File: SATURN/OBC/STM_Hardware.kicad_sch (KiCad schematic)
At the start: 6 parts, among them J1 SWD Pins, P1 USB_C_Plug, U1 STM32H735AGIx

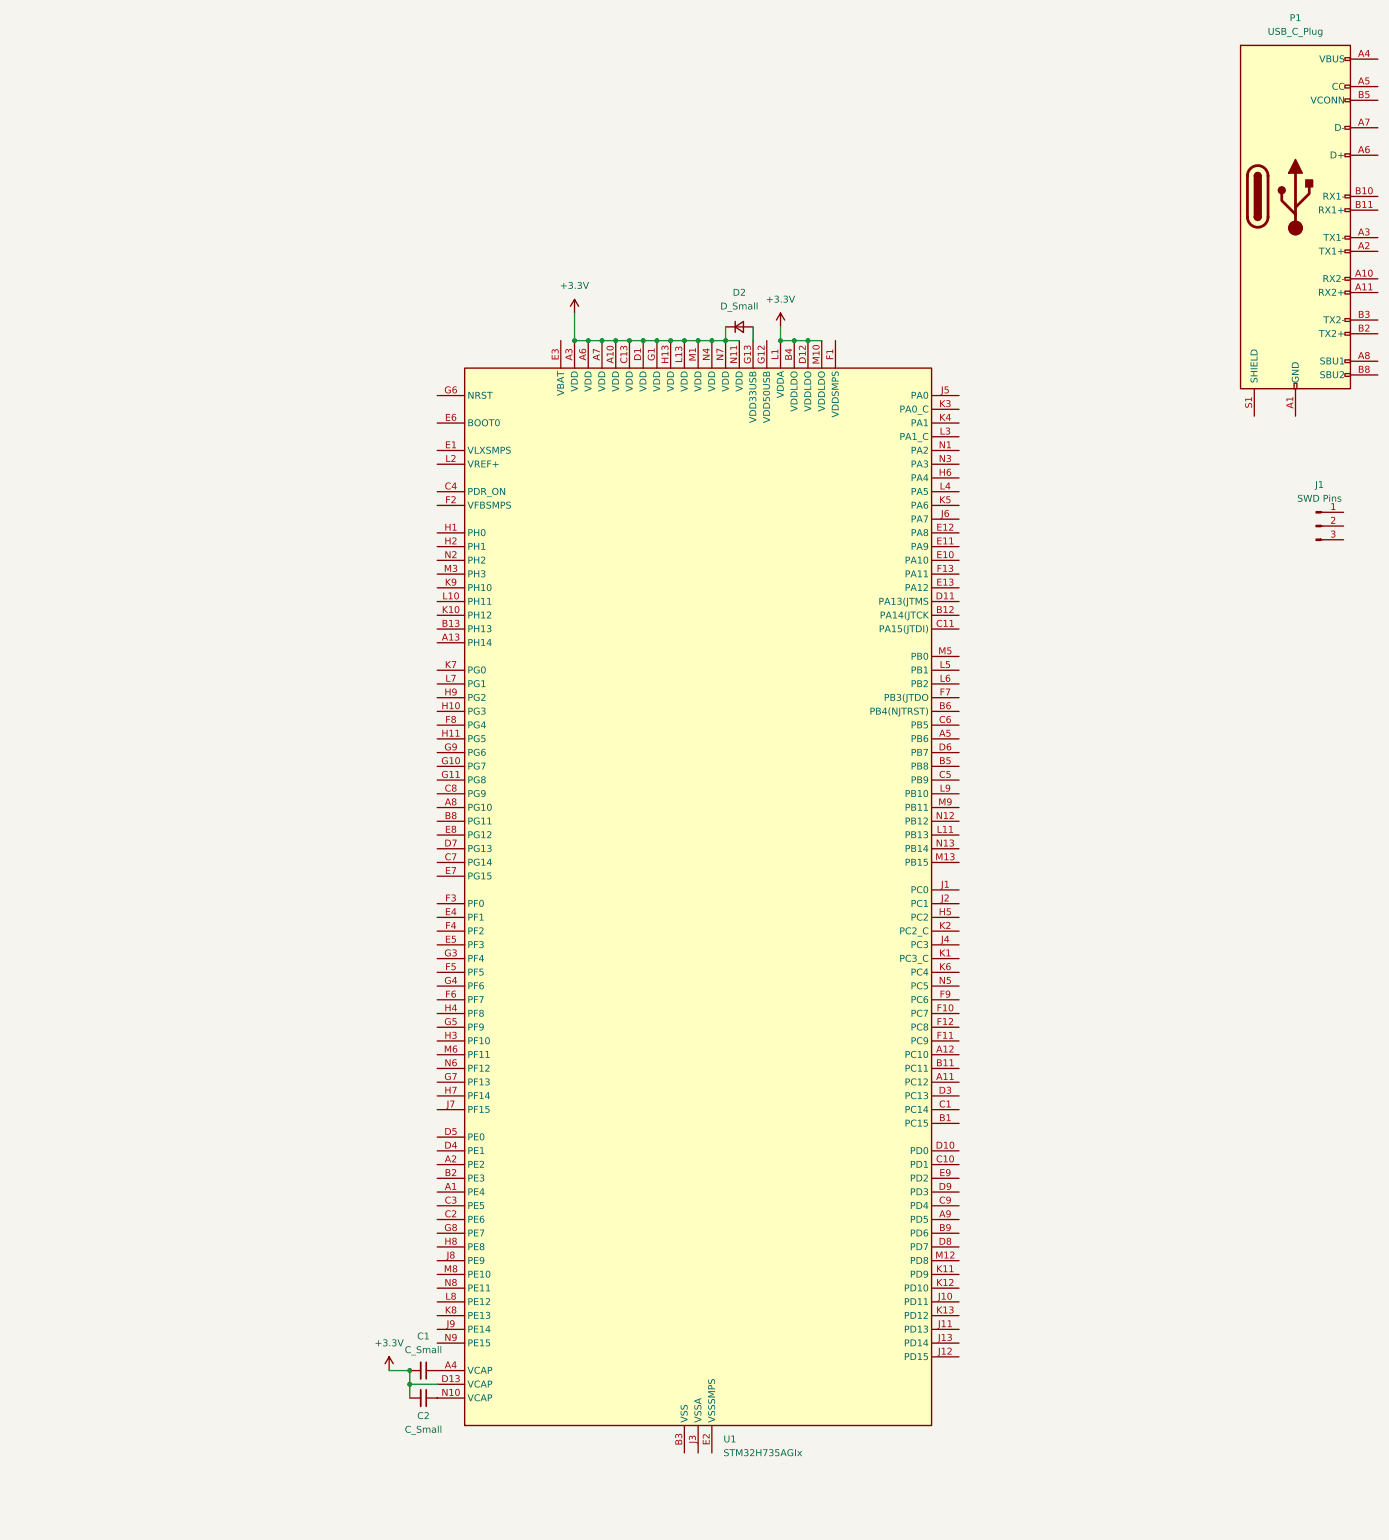
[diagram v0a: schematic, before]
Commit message: Working on STUFF(tm)
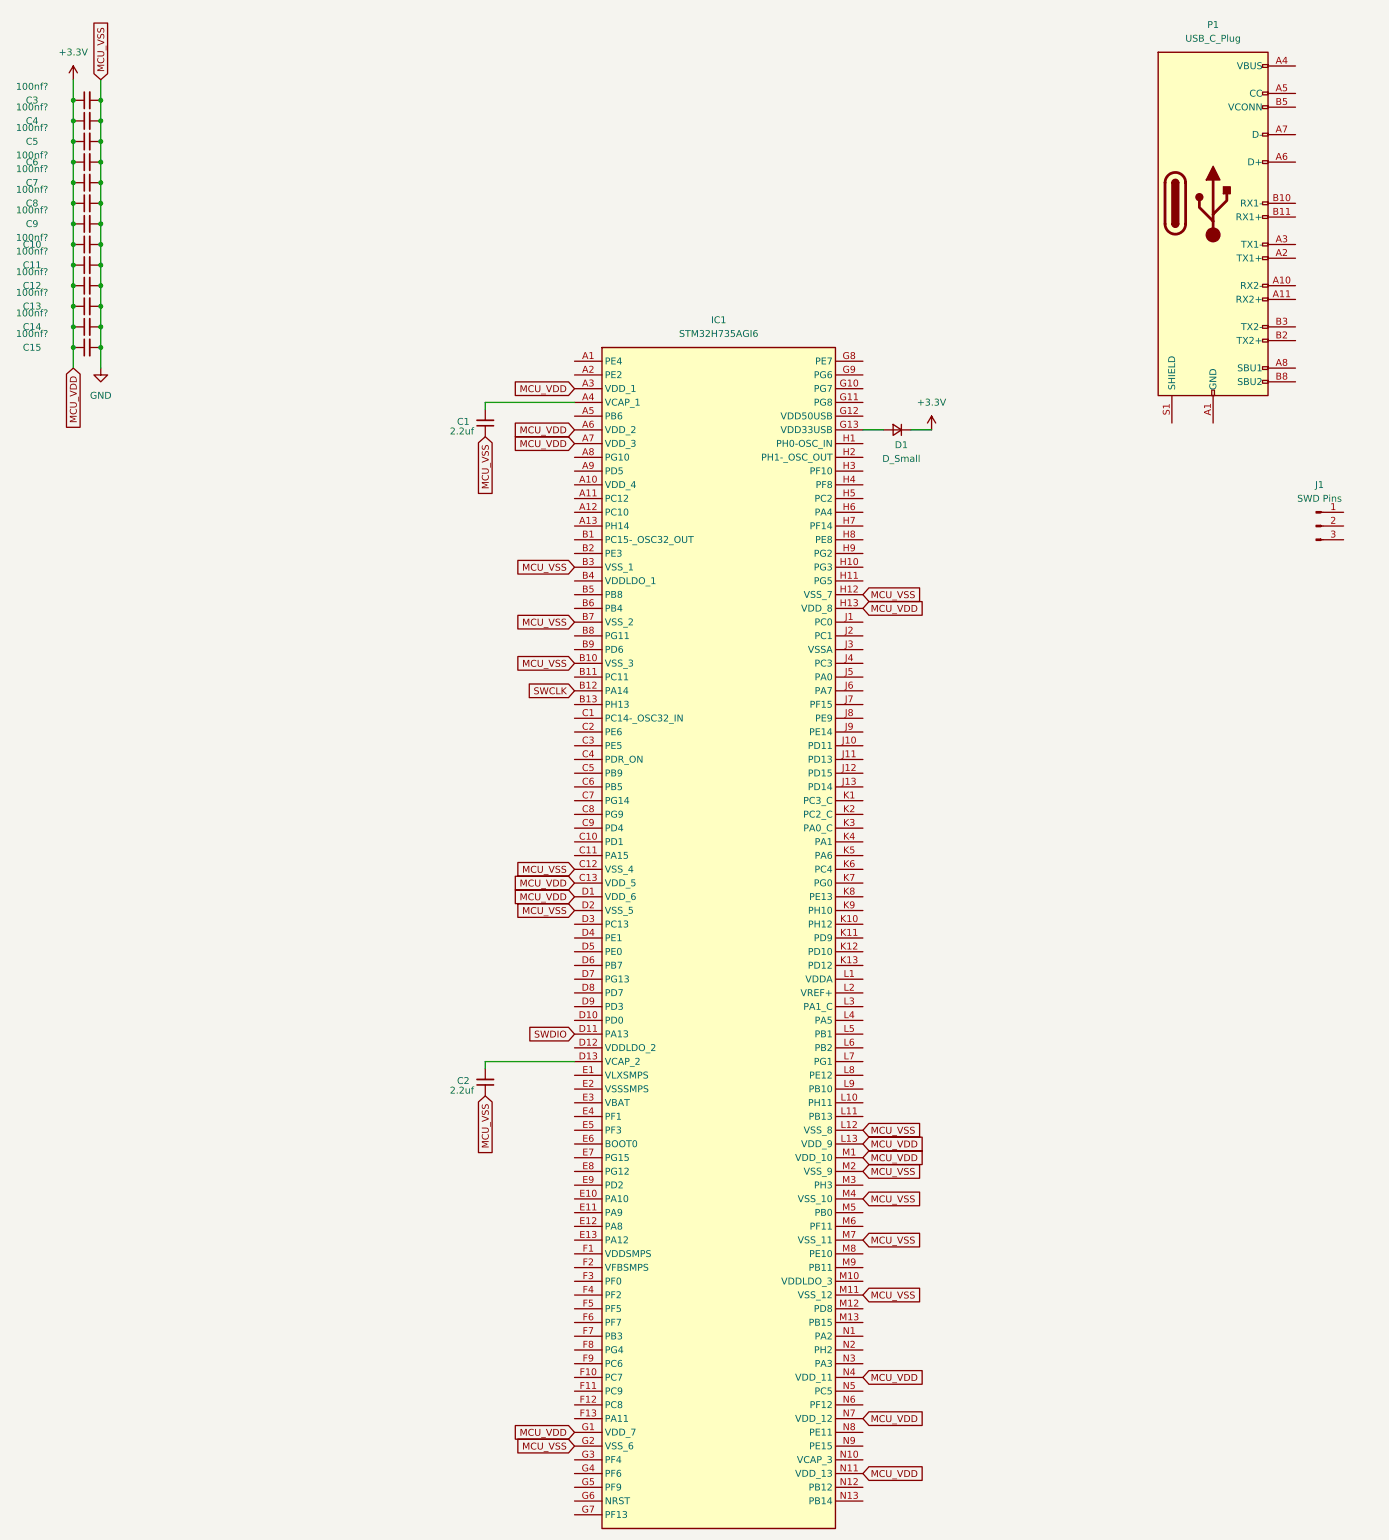
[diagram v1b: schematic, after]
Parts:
- removed U1: STM32H735AGIx, Package_BGA:UFBGA-169_7x7mm_Layout13x13_P0.5mm, symbol MCU_ST_STM32H7:STM32H735AGIx
- added C10, C11, C12, C13, C14, C15, C3, C4, C5, C6, C7, C8, C9: 100nf?, symbol Device:C_Small
- added IC1: STM32H735AGI6, BGA169C50P13X13_700X700X60, symbol STM32H735AGI6:STM32H735AGI6
- C1, C2: value C_Small -> 2.2uf
- renumbered D2 to D1
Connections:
- net +3.3V: now also C10.1, C11.1, C12.1, C13.1, C14.1, C15.1, C3.1, C4.1, C5.1, C6.1, C7.1, C8.1, C9.1, IC1.A3 (VDD_1), IC1.A6 (VDD_2), IC1.A7 (VDD_3), IC1.C13 (VDD_5), IC1.D1 (VDD_6), IC1.G1 (VDD_7), IC1.H13 (VDD_8), IC1.L13 (VDD_9), IC1.M1 (VDD_10), IC1.N11 (VDD_13), IC1.N4 (VDD_11), IC1.N7 (VDD_12); no longer C1.2, C2.2
- net at D1.2 (A): now also IC1.G13 (VDD33USB)
- net GND: now reaches C1.1
- net GND: now also C2.1, C10.2, C11.2, C12.2, C13.2, C14.2, C15.2, C3.2, C4.2, C5.2, C6.2, C7.2, C8.2, C9.2, IC1.B10 (VSS_3), IC1.B3 (VSS_1), IC1.B7 (VSS_2), IC1.C12 (VSS_4), IC1.D2 (VSS_5), IC1.G2 (VSS_6), IC1.H12 (VSS_7), IC1.L12 (VSS_8), IC1.M11 (VSS_12), IC1.M2 (VSS_9), IC1.M4 (VSS_10), IC1.M7 (VSS_11)
- new net: C2.2, IC1.D13 (VCAP_2)
- new net: C1.2, IC1.A4 (VCAP_1)
- new net SWCLK: IC1.B12 (PA14)
- new net SWDIO: IC1.D11 (PA13)
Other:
- moved on the sheet: C1, D1, P1
